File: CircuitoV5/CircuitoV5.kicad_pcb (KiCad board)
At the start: 2 copper layers, 34 x 45 mm, 18 parts, among them J1 Conn_01x05, J2 Screw_Terminal_01x02, J3 Screw_Terminal_01x02, U1 LM324, U2 LM358

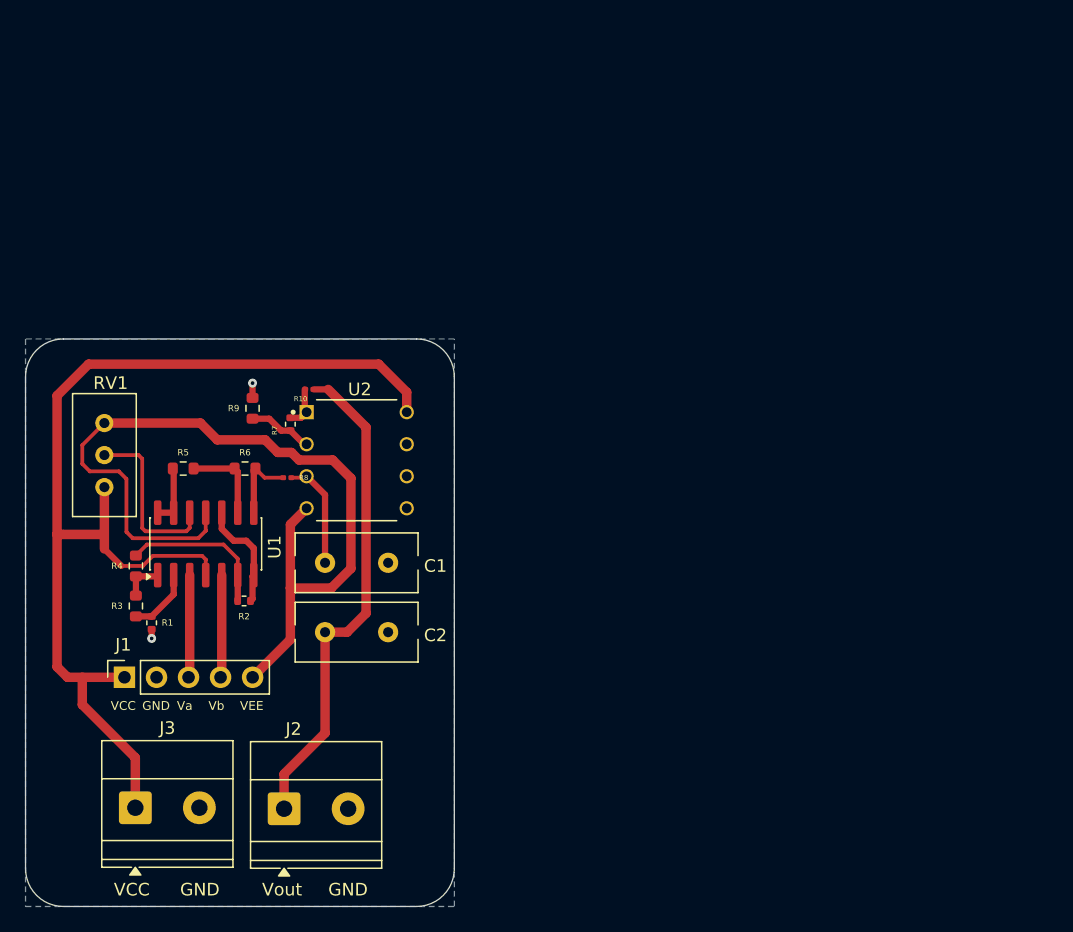
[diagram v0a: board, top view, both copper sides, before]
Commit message: Routed and done
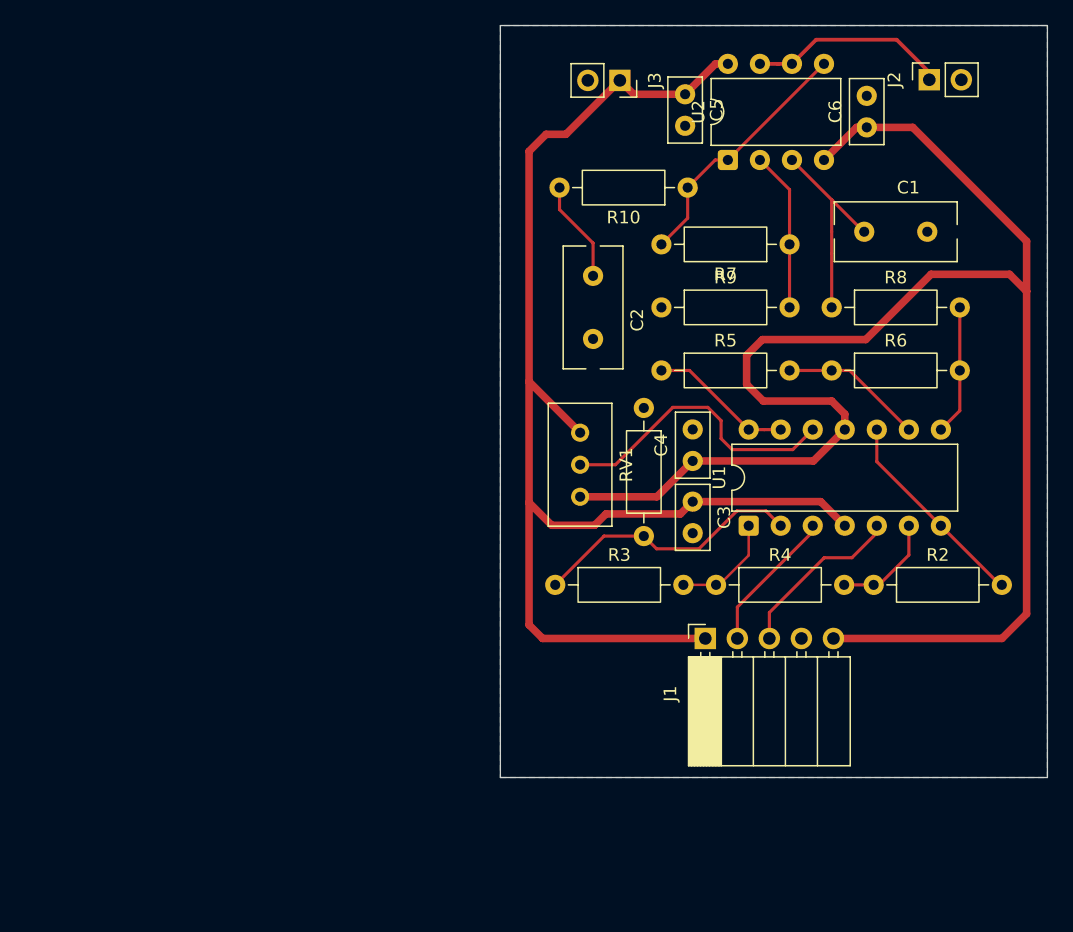
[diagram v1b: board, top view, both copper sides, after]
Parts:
- added C3: LM324, Capacitor_THT:C_Disc_D5.0mm_W2.5mm_P2.50mm, F.Cu at (92.9, 77.9)
- added C4: LM324, Capacitor_THT:C_Disc_D5.0mm_W2.5mm_P2.50mm, F.Cu at (92.9, 74.7)
- added C5: LM358, Capacitor_THT:C_Disc_D5.0mm_W2.5mm_P2.50mm, F.Cu at (92.3, 45.6)
- added C6: LM358, Capacitor_THT:C_Disc_D5.0mm_W2.5mm_P2.50mm, F.Cu at (106.7, 48.2)
- J1: footprint Connector_PinSocket_2.54mm:PinSocket_1x05_P2.54mm_Vertical -> Connector_PinSocket_2.54mm:PinSocket_1x05_P2.54mm_Horizontal
- J2, J3: value Screw_Terminal_01x02 -> Conn_01x02; footprint TerminalBlock_Phoenix:TerminalBlock_Phoenix_MKDS-1,5-2-5.08_1x02_P5.08mm_Horizontal -> Connector_PinSocket_2.54mm:PinSocket_1x02_P2.54mm_Vertical
- R1, R2, R7: footprint Resistor_SMD:R_0402_1005Metric -> Resistor_THT:R_Axial_DIN0207_L6.3mm_D2.5mm_P10.16mm_Horizontal
- R10, R8: footprint Resistor_SMD:R_0201_0603Metric -> Resistor_THT:R_Axial_DIN0207_L6.3mm_D2.5mm_P10.16mm_Horizontal
- R3, R4, R5, R6, R9: footprint Resistor_SMD:R_0603_1608Metric -> Resistor_THT:R_Axial_DIN0207_L6.3mm_D2.5mm_P10.16mm_Horizontal
- U1: footprint Package_SO:SOIC-14_3.9x8.7mm_P1.27mm -> Package_DIP:DIP-14_W7.62mm
- U2: footprint footprints:DIP794W45P254L959H508Q8 -> Package_DIP:DIP-8_W7.62mm
- moved J2 77.2 mm to (111.7, 44.5), turned to 90 degrees
- moved J3 69.3 mm to (87.1, 44.5), turned to -90 degrees
- moved C1 50.2 mm to (105.0, 56.5)
- moved R2 49.9 mm to (107.2, 84.5)
- moved R6 47.2 mm to (103.9, 67.5)
- moved J1 46.2 mm to (93.9, 88.8)
- moved R4 46.0 mm to (94.8, 84.5), turned to 0 degrees
- moved R8 45.2 mm to (103.9, 62.5), turned to 0 degrees
- moved U1 43.1 mm to (97.3, 79.8)
- moved R1 42.6 mm to (89.0, 70.5), turned to -90 degrees
- moved R7 42.1 mm to (100.6, 57.5), turned to 180 degrees
- moved R5 38.7 mm to (90.4, 67.5)
- moved RV1 38.2 mm to (84.0, 77.5), turned to -90 degrees
- moved U2 37.9 mm to (95.7, 50.8), turned to 90 degrees
- moved C2 37.5 mm to (85.0, 58.5), turned to -90 degrees
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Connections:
- C2 pad 1: /Vout -> Net-(C2-Pad1)
- J1 pad 2: GND -> /Va
- J1 pad 3: /Va -> /Vb
- J1 pad 4: /Vb -> GND
- R10 pad 1: Net-(R10-Pad1) -> Net-(U2B-+)
- R10 pad 2: /Vout -> Net-(C2-Pad1)
- R7 pad 2: Net-(R10-Pad1) -> Net-(U2B-+)
- U2 pad 1: Net-(R10-Pad1) -> Net-(U2B-+)
- U2 pad 5: unconnected-(U2B-+-Pad5) -> Net-(U2B-+)
- U2 pad 6: unconnected-(U2B---Pad6) -> /Vout
- U2 pad 7: unconnected-(U2-Pad7) -> /Vout
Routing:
- net VEE: track 69.5 -> 127.5 mm
- net /Vout: track 40.1 -> 15.9 mm
- net Net-(U2B-+): track 0.00 -> 20.2 mm
- net Net-(U1A--): track 5.25 -> 21.6 mm
- net VCC: track 89.5 -> 104.6 mm
- net Net-(U1D-+): track 13.8 -> 23.2 mm
- net Net-(C2-Pad1): track 0.00 -> 8.10 mm
- net Net-(U2A-+): track 8.73 -> 16.6 mm
- net Net-(U1C-+): track 8.75 -> 16.5 mm
- net Net-(U2A--): track 5.12 -> 12.7 mm
- net Net-(U1D--): track 4.80 -> 11.4 mm
- net /Vb: track 8.14 -> 13.8 mm
- net Net-(R3-Pad2): track 3.29 -> 8.50 mm
- net Net-(U1C--): track 6.85 -> 11.4 mm
- net Net-(R6-Pad2): track 6.06 -> 10.3 mm
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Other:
- board size 34 x 45 mm -> 43.4 x 59.6 mm
- board text removed: "GND"
- board text removed: "VCC"
- board text removed: "VEE"
- board text removed: "Va"
- board text removed: "Vb"
- board text removed: "Vout"
